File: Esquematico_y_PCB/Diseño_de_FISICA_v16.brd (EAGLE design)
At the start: 100 x 80 mm, 39 parts, among them IC1 2133-DRV8825, IC2 2133-DRV8825, IC3 2133-DRV8825, J2 3A/250V

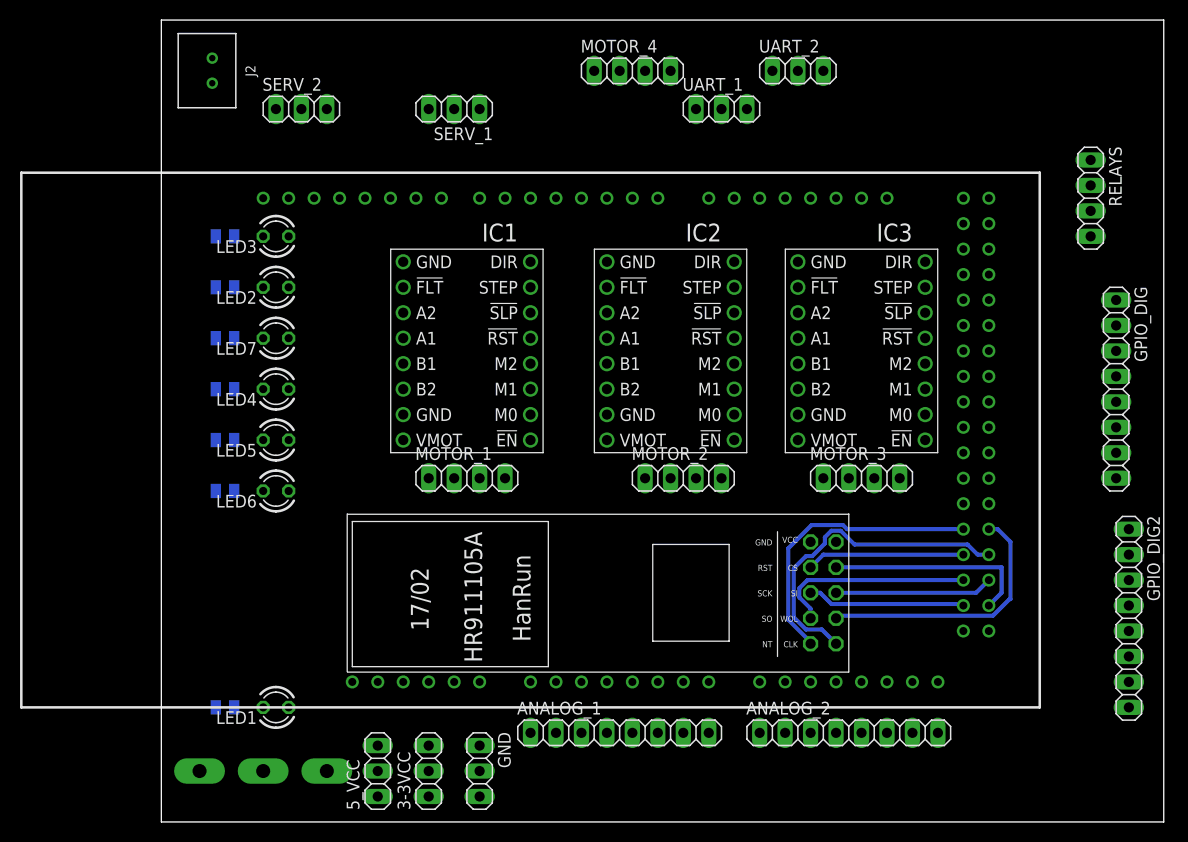
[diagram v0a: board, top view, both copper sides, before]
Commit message: Acualización PCB y SCH
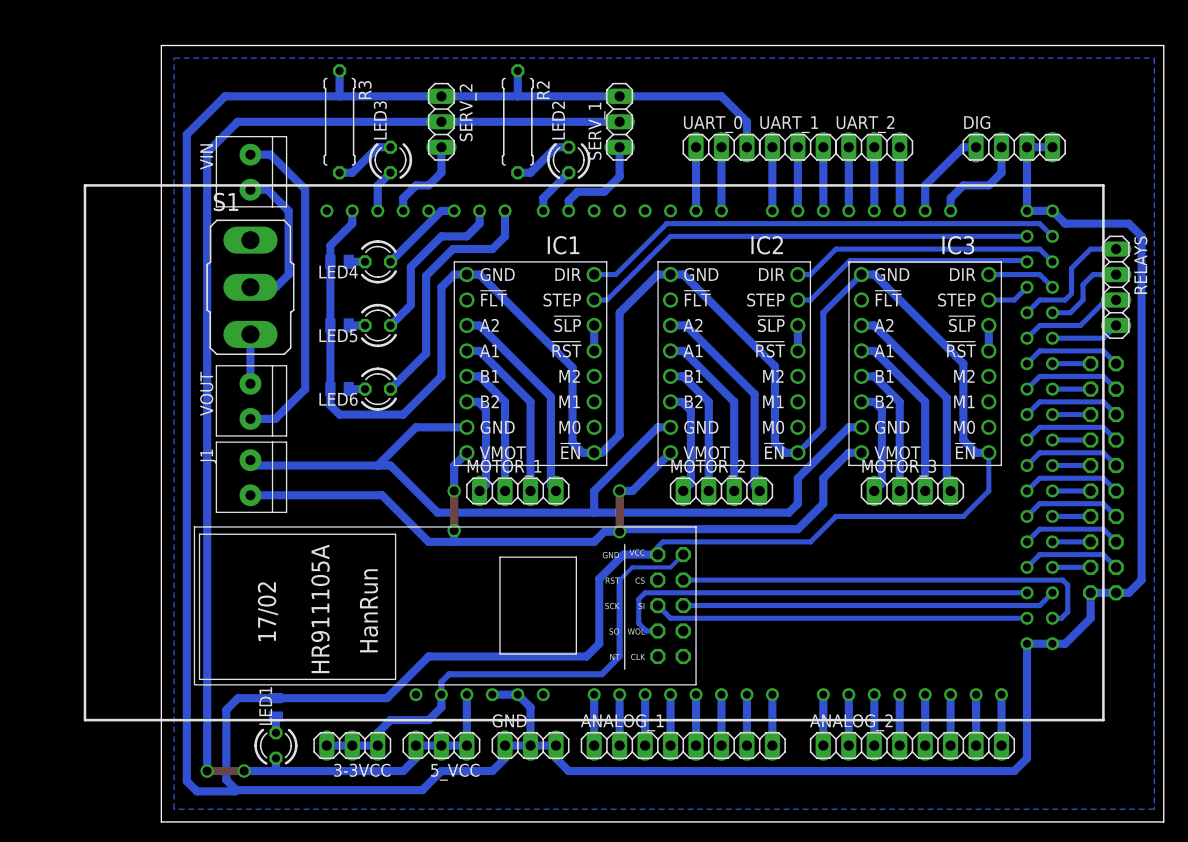
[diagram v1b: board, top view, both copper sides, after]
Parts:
- removed GPIO_DIG2: PINHD-1X8, Connector:1X08
- removed J2: 3A/250V, Connector:B2B-XH-A
- removed JP1, JP2, JP3: (no value), adafruit:1X1-BIGPOGO
- removed LED7: (no value), led:LED3MM
- removed MOTOR_4: PINHD-1X4, Connector:1X04
- removed R7: (no value), Resistor:RESC2012X65
- added DIG: PINHD-1X4, Connector:1X04
- added J1, VIN, VOUT: 1X2-3.5MM, adafruit:1X2-3.5MM
- added S1: (no value), switch:M9040P
- added UART_0: PINHD-1X3, Connector:1X03
- GPIO_DIG: value PINHD-1X8 -> (none); device Connector:1X08 -> pinhead:2X10
- R2, R3: device Resistor:RESC2012X65 -> rcl:0309/10
- moved R2 33.6 mm to (35.6, 69.8), flipped to the top, turned to 270 degrees
- moved LED2 31.9 mm to (40.6, 66.0), turned to 90 degrees
- moved R4 17.1 mm to (17.8, 55.9)
- moved SERV_1 16.6 mm to (45.7, 69.8), turned to 90 degrees
- moved LED4 16.3 mm to (21.6, 55.9)
- moved R5 16.2 mm to (17.8, 49.5)
- moved R3 16.2 mm to (17.8, 69.8), flipped to the top, turned to 270 degrees
- moved LED5 15.3 mm to (21.6, 49.5)
- moved R6 15.3 mm to (17.8, 43.2)
- moved MODULO_ETHERNET 15.3 mm to (53.3, 19.1)
- moved LED6 14.4 mm to (21.6, 43.2)
- moved SERV_2 14.0 mm to (27.9, 69.8), turned to 270 degrees
- moved LED3 13.7 mm to (22.9, 66.0), turned to 90 degrees
- moved UART_2 10.8 mm to (71.1, 67.3)
- moved RELAYS 9.25 mm to (95.2, 53.3)
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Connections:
- removed net AREF: ARDUINOMEGA2560.AREF, MOTOR_4.4
- removed net GND1: IC1.9, IC2.9, IC3.9
- removed net LED_AUX: ARDUINOMEGA2560.11, LED7.A
- removed net N$37: LED7.K, R7.2
- removed net RST: ARDUINOMEGA2560.RESET, MOTOR_4.3
- removed net VCC: J2.1, JP1.P$1, SERV_1.2, SERV_2.2
- new net GND_MOT: IC1.15, IC2.15, IC3.15, J1.1
- new net N$1: S1.2, VIN.2
- new net N$2: S1.3, VOUT.1
- new net N$3: VIN.1, VOUT.2
- net CLK: now also GPIO_DIG.18; no longer MODULO_ETHERNET.CLK
- net D20: now also DIG.1; no longer GPIO_DIG2.7
- net D21: now also DIG.2; no longer GPIO_DIG2.8
- net D40: now also GPIO_DIG.9; no longer GPIO_DIG2.1
- net D41: now also GPIO_DIG.10; no longer GPIO_DIG2.2
- net D42: now also GPIO_DIG.11; no longer GPIO_DIG2.3
- net D43: now also GPIO_DIG.12; no longer GPIO_DIG2.4
- net D44: now also GPIO_DIG.13; no longer GPIO_DIG2.5
- net D45: now also GPIO_DIG.14; no longer GPIO_DIG2.6
- net GND: now also DIG.3, DIG.4, GPIO_DIG.19, GPIO_DIG.20, IC1.1, IC1.9, IC2.1, IC2.9, IC3.1, IC3.9, UART_0.3; no longer IC1.15, IC2.15, IC3.15, J2.2, JP3.P$1, R7.1
- net LED_SERV_1: now also ARDUINOMEGA2560.7; no longer ARDUINOMEGA2560.12
- net NT: now also GPIO_DIG.15; no longer MODULO_ETHERNET.NT
- net PWM_SERV_2: now also ARDUINOMEGA2560.12; no longer ARDUINOMEGA2560.7
- net RST_1: now also GPIO_DIG.17; no longer MODULO_ETHERNET.RST
- net RX: now also UART_0.2; no longer MOTOR_4.2
- net TX: now also UART_0.1; no longer MOTOR_4.1
- net VCC_5: now also SERV_1.2, SERV_2.2; no longer JP2.P$1
- net VCC_MOT: now also J1.2
- net WOL: now also GPIO_DIG.16; no longer MODULO_ETHERNET.WOL
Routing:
- net GND: track 0.00 -> 573.6 mm
- net VCC_5: track 0.00 -> 138.2 mm, vias 0 -> 2
- net GND_MOT: track 0.00 -> 91.0 mm
- net VCC_MOT: track 0.00 -> 88.2 mm, vias 0 -> 4
- net VCC_3_3: track 0.00 -> 50.1 mm
- net DIR_1: track 0.00 -> 48.4 mm
- net STEP_1: track 0.00 -> 45.8 mm
- net N$3: track 0.00 -> 33.5 mm
- net CLK: track 32.6 -> 3.81 mm
- net DIR_2: track 0.00 -> 27.0 mm
- net LED_MOT_1: track 0.00 -> 24.8 mm
- net STEP_2: track 0.00 -> 24.5 mm
- net SO: track 20.2 -> 43.6 mm
- net WOL: track 26.6 -> 3.81 mm
- net CS: track 20.8 -> 43.0 mm
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- added copper zone on layer 16, net GND
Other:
- board size 100 x 80 mm -> 100 x 77.5 mm
